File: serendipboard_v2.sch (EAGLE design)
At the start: 29 parts, among them IC1 TP4056, IC2 DW01A, IC3 DS3231/SO, Q1 FS8205A, Q2 DMP3056LSD, U1 MAX17043, U2 AP2112-3.3, U3 AP2112-3.3

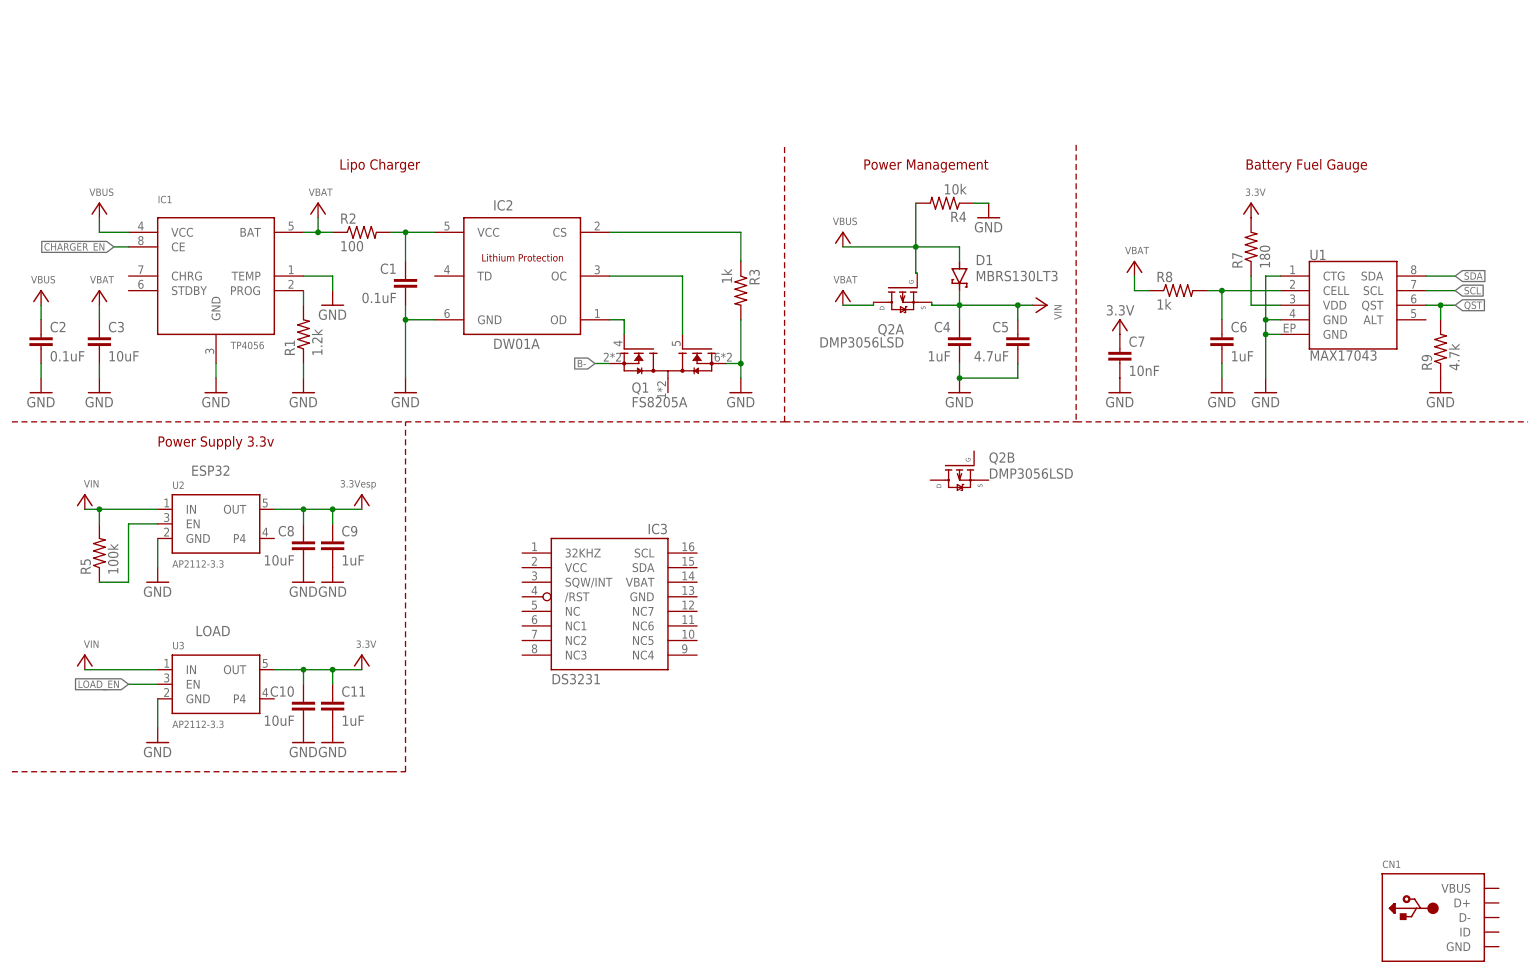
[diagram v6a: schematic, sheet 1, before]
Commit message: Update serendipboard_v2.sch
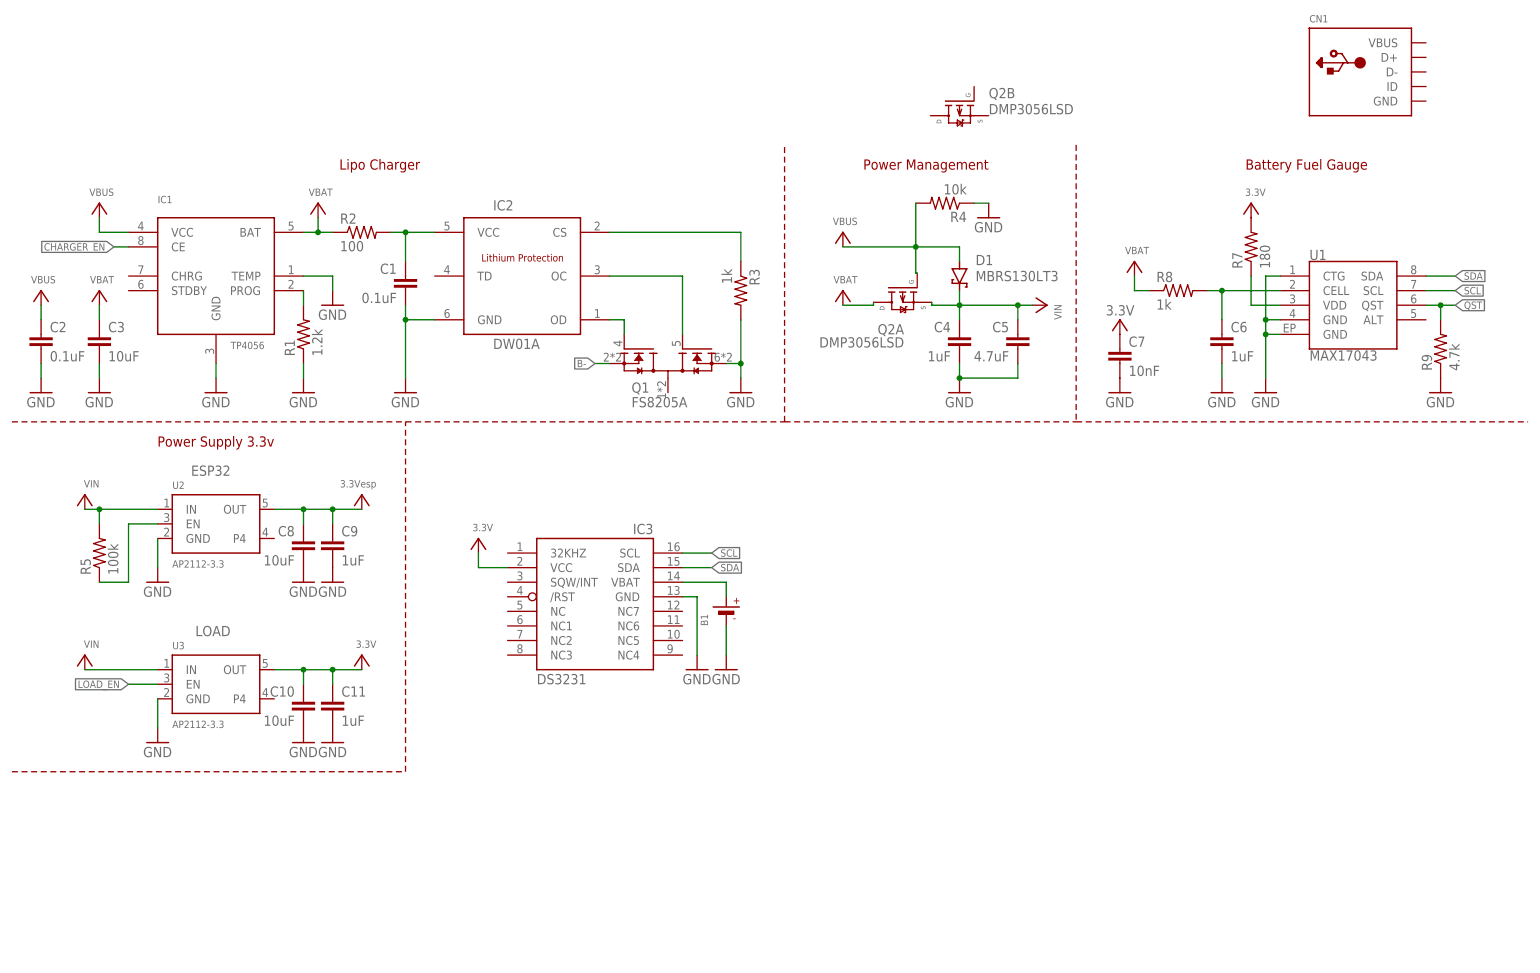
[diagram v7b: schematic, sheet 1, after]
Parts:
- added B1: (no value), microbuilder:BATTERYCR1220_SMT
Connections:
- new net N$9: B1.+, IC3.VBAT
- net GND: now also B1.-, IC3.GND
- net SCL: now also IC3.SCL
- net SDA: now also IC3.SDA
- net VCC: now also IC3.VCC
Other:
- moved on the sheet: CN1, IC3, Q2B
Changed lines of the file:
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@@
 <part name="P+11" library="supply1" library_urn="urn:adsk.eagle:library:371" deviceset="VCC" device="" value="3.3V"/>
 <part name="IC3" library="DS3231" deviceset="DS3231" device="/SO"/>
+<part name="P+15" library="supply1" library_urn="urn:adsk.eagle:library:371" deviceset="VCC" device="" value="3.3V"/>
+<part name="B1" library="microbuilder" deviceset="BATTERY" device="CR1220_SMT"/>
+<part name="GND20" library="supply1" library_urn="urn:adsk.eagle:library:371" deviceset="GND" device=""/>
+<part name="GND21" library="supply1" library_urn="urn:adsk.eagle:library:371" deviceset="GND" device=""/>
 </parts>
 <sheets>
@@
 <text x="38.1" y="124.46" size="1.778" layer="95" rot="R180">ESP32</text>
 <text x="38.1" y="96.52" size="1.778" layer="95" rot="R180">LOAD</text>
-<wire x1="0" y1="71.12" x2="66.04" y2="71.12" width="0.1524" layer="94" style="shortdash"/>
-<wire x1="66.04" y1="71.12" x2="68.58" y2="71.12" width="0.1524" layer="94" style="shortdash"/>
+<wire x1="0" y1="71.12" x2="68.58" y2="71.12" width="0.1524" layer="94" style="shortdash"/>
 <wire x1="68.58" y1="71.12" x2="68.58" y2="132.08" width="0.1524" layer="94" style="shortdash"/>
 </plain>
@@
 <attribute name="VALUE" x="124.46" y="134.62" size="1.778" layer="96"/>
 </instance>
-<instance part="CN1" gate="G$1" x="248.92" y="45.72" smashed="yes">
-<attribute name="NAME" x="238.76" y="54.356" size="1.27" layer="95"/>
-<attribute name="VALUE" x="238.76" y="35.56" size="1.27" layer="96"/>
+<instance part="CN1" gate="G$1" x="236.22" y="193.04" smashed="yes">
+<attribute name="NAME" x="226.06" y="201.676" size="1.27" layer="95"/>
+<attribute name="VALUE" x="226.06" y="182.88" size="1.27" layer="96"/>
 </instance>
 <instance part="C3" gate="G$1" x="15.24" y="147.32" smashed="yes">
@@
 <attribute name="NAME" x="155.448" y="149.098" size="1.778" layer="95" rot="R180"/>
 </instance>
-<instance part="Q2" gate="B" x="165.1" y="124.46" smashed="yes" rot="R270">
-<attribute name="VALUE" x="170.18" y="123.952" size="1.778" layer="96" align="top-left"/>
-<attribute name="NAME" x="170.18" y="124.968" size="1.778" layer="95"/>
+<instance part="Q2" gate="B" x="165.1" y="187.96" smashed="yes" rot="R270">
+<attribute name="VALUE" x="170.18" y="187.452" size="1.778" layer="96" align="top-left"/>
+<attribute name="NAME" x="170.18" y="188.468" size="1.778" layer="95"/>
 </instance>
 <instance part="R4" gate="G$1" x="162.56" y="170.18" smashed="yes" rot="R180">
@@
 <attribute name="VALUE" x="63.5" y="93.98" size="1.27" layer="96" rot="R180"/>
 </instance>
-<instance part="IC3" gate="G$1" x="104.14" y="99.06" smashed="yes">
-<attribute name="NAME" x="114.3" y="114.3" size="1.778" layer="95" rot="R180"/>
+<instance part="IC3" gate="G$1" x="101.6" y="99.06" smashed="yes">
+<attribute name="NAME" x="111.76" y="114.3" size="1.778" layer="95" rot="R180"/>
+</instance>
+<instance part="P+15" gate="VCC" x="81.28" y="111.76" smashed="yes">
+<attribute name="VALUE" x="83.82" y="114.3" size="1.27" layer="96" rot="R180"/>
+</instance>
+<instance part="B1" gate="G$1" x="124.46" y="99.06" smashed="yes" rot="R90">
+<attribute name="NAME" x="121.285" y="96.52" size="1.27" layer="95" rot="R90"/>
+<attribute name="VALUE" x="129.54" y="96.52" size="1.27" layer="96" rot="R90"/>
+</instance>
+<instance part="GND20" gate="1" x="119.38" y="88.9" smashed="yes">
+<attribute name="VALUE" x="116.84" y="86.36" size="1.778" layer="96"/>
+</instance>
+<instance part="GND21" gate="1" x="124.46" y="88.9" smashed="yes">
+<attribute name="VALUE" x="121.92" y="86.36" size="1.778" layer="96"/>
 </instance>
 </instances>
@@
 <pinref part="U3" gate="G$1" pin="GND"/>
 <wire x1="25.4" y1="78.74" x2="25.4" y2="83.82" width="0.1524" layer="91"/>
+</segment>
+<segment>
+<pinref part="IC3" gate="G$1" pin="GND"/>
+<pinref part="GND20" gate="1" pin="GND"/>
+<wire x1="116.84" y1="101.6" x2="119.38" y2="101.6" width="0.1524" layer="91"/>
+<wire x1="119.38" y1="101.6" x2="119.38" y2="91.44" width="0.1524" layer="91"/>
+</segment>
+<segment>
+<pinref part="B1" gate="G$1" pin="-"/>
+<pinref part="GND21" gate="1" pin="GND"/>
+<wire x1="124.46" y1="96.52" x2="124.46" y2="91.44" width="0.1524" layer="91"/>
 </segment>
 </net>
@@
 <pinref part="P+11" gate="VCC" pin="VCC"/>
 </segment>
+<segment>
+<pinref part="IC3" gate="G$1" pin="VCC"/>
+<pinref part="P+15" gate="VCC" pin="VCC"/>
+<wire x1="81.28" y1="109.22" x2="81.28" y2="106.68" width="0.1524" layer="91"/>
+<wire x1="81.28" y1="106.68" x2="86.36" y2="106.68" width="0.1524" layer="91"/>
+</segment>
 </net>
 <net name="CHARGER_EN" class="0">
@@
 <label x="251.46" y="157.48" size="1.27" layer="95" xref="yes"/>
 </segment>
+<segment>
+<pinref part="IC3" gate="G$1" pin="SDA"/>
+<wire x1="116.84" y1="106.68" x2="121.92" y2="106.68" width="0.1524" layer="91"/>
+<label x="121.92" y="106.68" size="1.27" layer="95" xref="yes"/>
+</segment>
 </net>
 <net name="SCL" class="0">
@@
 <wire x1="246.38" y1="154.94" x2="251.46" y2="154.94" width="0.1524" layer="91"/>
 <label x="251.46" y="154.94" size="1.27" layer="95" xref="yes"/>
+</segment>
+<segment>
+<pinref part="IC3" gate="G$1" pin="SCL"/>
+<wire x1="116.84" y1="109.22" x2="121.92" y2="109.22" width="0.1524" layer="91"/>
+<label x="121.92" y="109.22" size="1.27" layer="95" xref="yes"/>
 </segment>
 </net>
@@
 </segment>
 </net>
+<net name="N$9" class="0">
+<segment>
+<pinref part="IC3" gate="G$1" pin="VBAT"/>
+<pinref part="B1" gate="G$1" pin="+"/>
+<wire x1="116.84" y1="104.14" x2="124.46" y2="104.14" width="0.1524" layer="91"/>
+<wire x1="124.46" y1="104.14" x2="124.46" y2="101.6" width="0.1524" layer="91"/>
+</segment>
+</net>

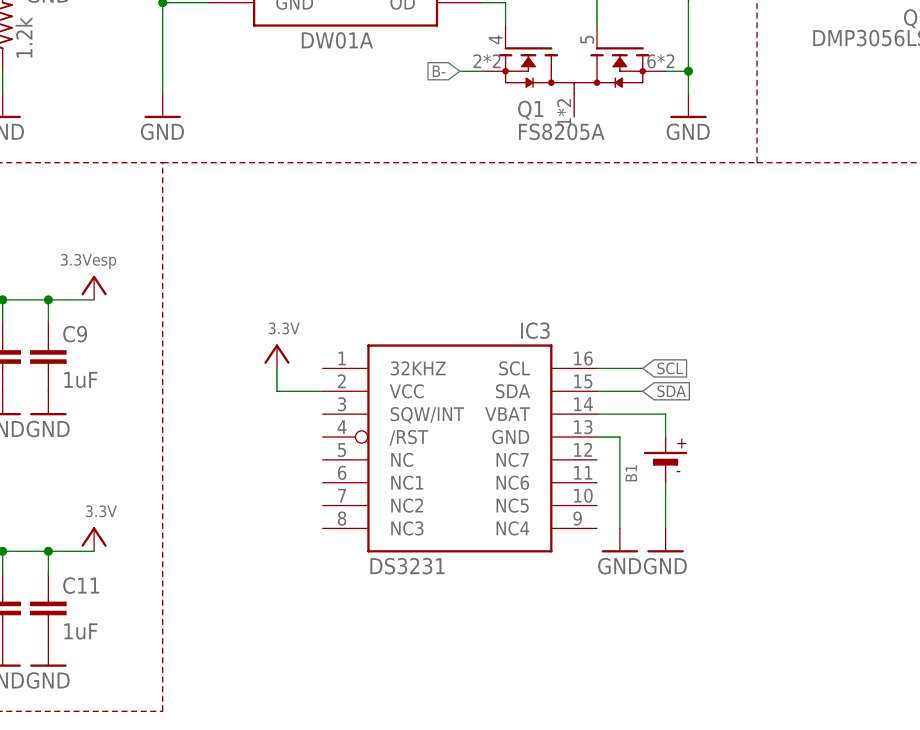
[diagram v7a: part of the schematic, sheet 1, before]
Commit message: Update serendipboard_v2.sch
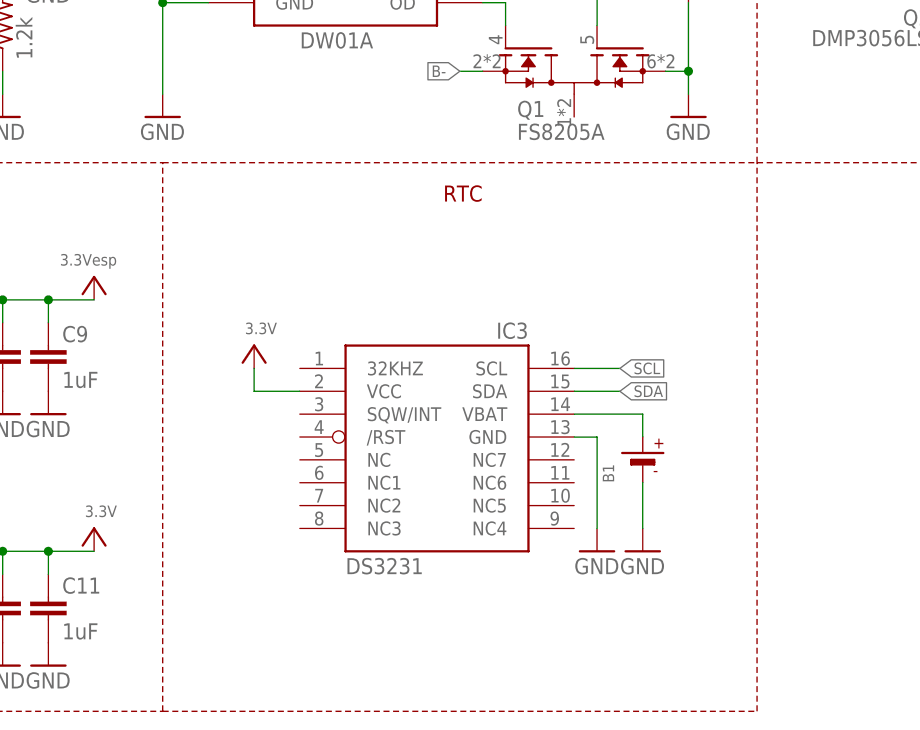
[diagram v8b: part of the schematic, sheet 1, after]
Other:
- note added: "RTC"
- moved on the sheet: B1, IC3
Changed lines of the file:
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@@
 <wire x1="0" y1="71.12" x2="68.58" y2="71.12" width="0.1524" layer="94" style="shortdash"/>
 <wire x1="68.58" y1="71.12" x2="68.58" y2="132.08" width="0.1524" layer="94" style="shortdash"/>
+<wire x1="68.58" y1="71.12" x2="134.62" y2="71.12" width="0.1524" layer="94" style="shortdash"/>
+<wire x1="134.62" y1="71.12" x2="134.62" y2="132.08" width="0.1524" layer="94" style="shortdash"/>
+<text x="104.14" y="129.54" size="1.778" layer="94" rot="R180">RTC</text>
 </plain>
 <instances>
@@
 <attribute name="VALUE" x="63.5" y="93.98" size="1.27" layer="96" rot="R180"/>
 </instance>
-<instance part="IC3" gate="G$1" x="101.6" y="99.06" smashed="yes">
-<attribute name="NAME" x="111.76" y="114.3" size="1.778" layer="95" rot="R180"/>
-</instance>
-<instance part="P+15" gate="VCC" x="81.28" y="111.76" smashed="yes">
-<attribute name="VALUE" x="83.82" y="114.3" size="1.27" layer="96" rot="R180"/>
-</instance>
-<instance part="B1" gate="G$1" x="124.46" y="99.06" smashed="yes" rot="R90">
-<attribute name="NAME" x="121.285" y="96.52" size="1.27" layer="95" rot="R90"/>
-<attribute name="VALUE" x="129.54" y="96.52" size="1.27" layer="96" rot="R90"/>
-</instance>
-<instance part="GND20" gate="1" x="119.38" y="88.9" smashed="yes">
-<attribute name="VALUE" x="116.84" y="86.36" size="1.778" layer="96"/>
-</instance>
-<instance part="GND21" gate="1" x="124.46" y="88.9" smashed="yes">
-<attribute name="VALUE" x="121.92" y="86.36" size="1.778" layer="96"/>
+<instance part="IC3" gate="G$1" x="99.06" y="99.06" smashed="yes">
+<attribute name="NAME" x="109.22" y="114.3" size="1.778" layer="95" rot="R180"/>
+</instance>
+<instance part="P+15" gate="VCC" x="78.74" y="111.76" smashed="yes">
+<attribute name="VALUE" x="81.28" y="114.3" size="1.27" layer="96" rot="R180"/>
+</instance>
+<instance part="B1" gate="G$1" x="121.92" y="99.06" smashed="yes" rot="R90">
+<attribute name="NAME" x="118.745" y="96.52" size="1.27" layer="95" rot="R90"/>
+<attribute name="VALUE" x="127" y="96.52" size="1.27" layer="96" rot="R90"/>
+</instance>
+<instance part="GND20" gate="1" x="116.84" y="88.9" smashed="yes">
+<attribute name="VALUE" x="114.3" y="86.36" size="1.778" layer="96"/>
+</instance>
+<instance part="GND21" gate="1" x="121.92" y="88.9" smashed="yes">
+<attribute name="VALUE" x="119.38" y="86.36" size="1.778" layer="96"/>
 </instance>
 </instances>
@@
 <pinref part="IC3" gate="G$1" pin="GND"/>
 <pinref part="GND20" gate="1" pin="GND"/>
-<wire x1="116.84" y1="101.6" x2="119.38" y2="101.6" width="0.1524" layer="91"/>
-<wire x1="119.38" y1="101.6" x2="119.38" y2="91.44" width="0.1524" layer="91"/>
+<wire x1="114.3" y1="101.6" x2="116.84" y2="101.6" width="0.1524" layer="91"/>
+<wire x1="116.84" y1="101.6" x2="116.84" y2="91.44" width="0.1524" layer="91"/>
 </segment>
 <segment>
 <pinref part="B1" gate="G$1" pin="-"/>
 <pinref part="GND21" gate="1" pin="GND"/>
-<wire x1="124.46" y1="96.52" x2="124.46" y2="91.44" width="0.1524" layer="91"/>
+<wire x1="121.92" y1="96.52" x2="121.92" y2="91.44" width="0.1524" layer="91"/>
 </segment>
 </net>
@@
 <pinref part="IC3" gate="G$1" pin="VCC"/>
 <pinref part="P+15" gate="VCC" pin="VCC"/>
-<wire x1="81.28" y1="109.22" x2="81.28" y2="106.68" width="0.1524" layer="91"/>
-<wire x1="81.28" y1="106.68" x2="86.36" y2="106.68" width="0.1524" layer="91"/>
+<wire x1="78.74" y1="109.22" x2="78.74" y2="106.68" width="0.1524" layer="91"/>
+<wire x1="78.74" y1="106.68" x2="83.82" y2="106.68" width="0.1524" layer="91"/>
 </segment>
 </net>
@@
 <segment>
 <pinref part="IC3" gate="G$1" pin="SDA"/>
-<wire x1="116.84" y1="106.68" x2="121.92" y2="106.68" width="0.1524" layer="91"/>
-<label x="121.92" y="106.68" size="1.27" layer="95" xref="yes"/>
+<wire x1="114.3" y1="106.68" x2="119.38" y2="106.68" width="0.1524" layer="91"/>
+<label x="119.38" y="106.68" size="1.27" layer="95" xref="yes"/>
 </segment>
 </net>
@@
 <segment>
 <pinref part="IC3" gate="G$1" pin="SCL"/>
-<wire x1="116.84" y1="109.22" x2="121.92" y2="109.22" width="0.1524" layer="91"/>
-<label x="121.92" y="109.22" size="1.27" layer="95" xref="yes"/>
+<wire x1="114.3" y1="109.22" x2="119.38" y2="109.22" width="0.1524" layer="91"/>
+<label x="119.38" y="109.22" size="1.27" layer="95" xref="yes"/>
 </segment>
 </net>
@@
 <pinref part="IC3" gate="G$1" pin="VBAT"/>
 <pinref part="B1" gate="G$1" pin="+"/>
-<wire x1="116.84" y1="104.14" x2="124.46" y2="104.14" width="0.1524" layer="91"/>
-<wire x1="124.46" y1="104.14" x2="124.46" y2="101.6" width="0.1524" layer="91"/>
-</segment>
-</net>
+<wire x1="114.3" y1="104.14" x2="121.92" y2="104.14" width="0.1524" layer="91"/>
+<wire x1="121.92" y1="104.14" x2="121.92" y2="101.6" width="0.1524" layer="91"/>
+</segment>
+</net>
